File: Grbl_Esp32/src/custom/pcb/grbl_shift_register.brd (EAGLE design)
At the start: 69 parts

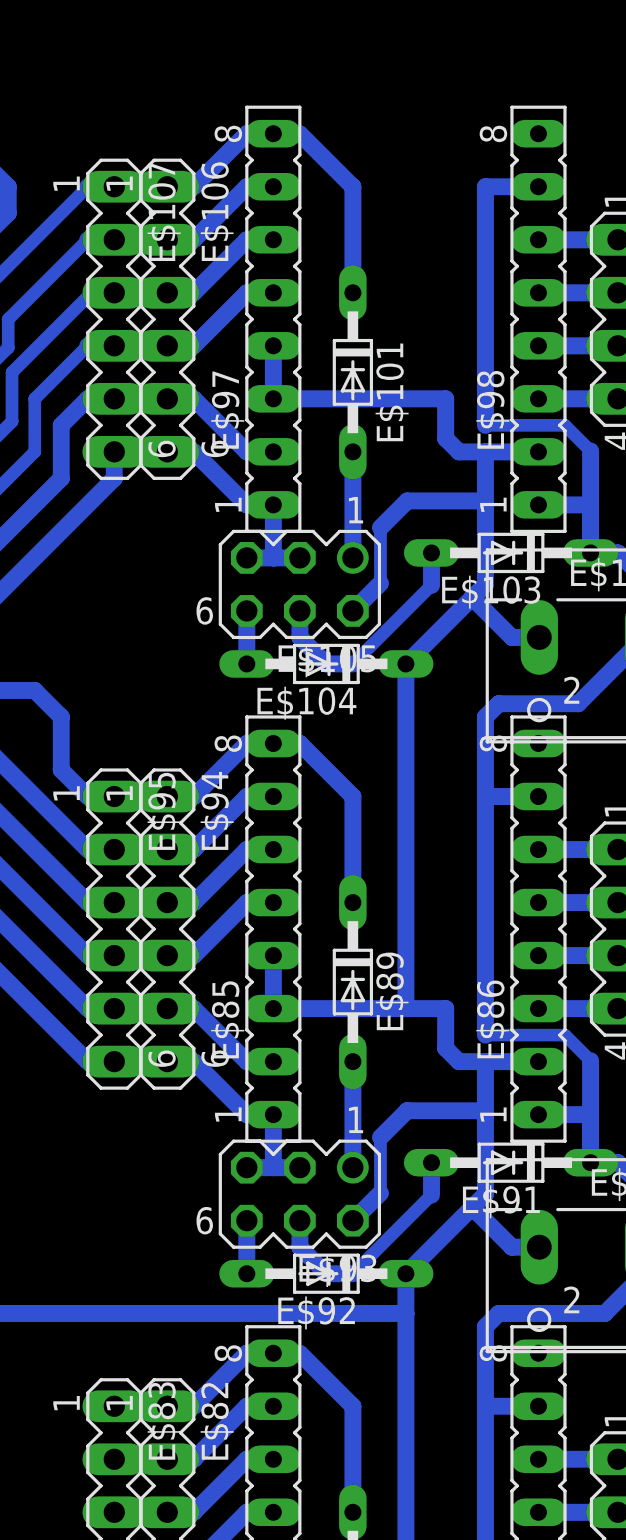
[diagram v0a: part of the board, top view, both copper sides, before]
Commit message: pcb
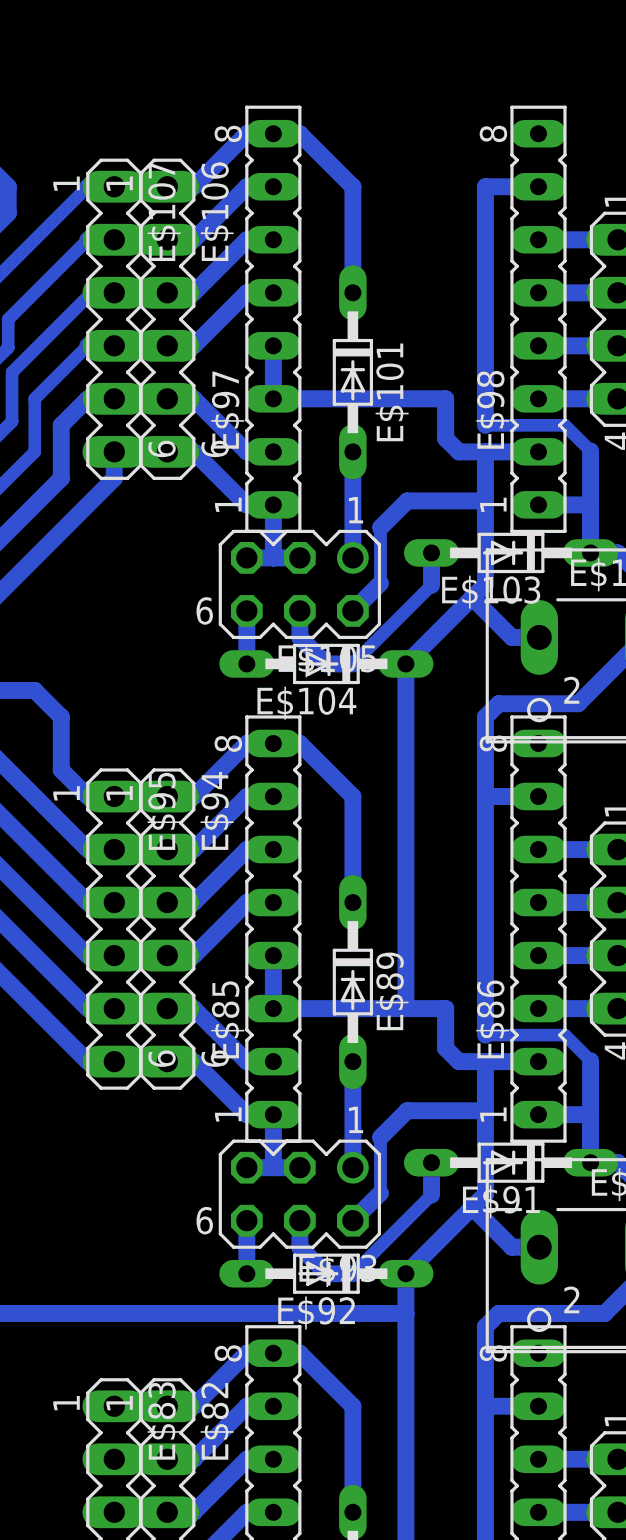
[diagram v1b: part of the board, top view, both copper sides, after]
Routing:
- net S$89: track 17.3 -> 18.6 mm
- net S$115: track 30.7 -> 32.0 mm
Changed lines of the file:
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@@
 <contactref element="E$77" pad="C"/>
 <contactref element="E$73" pad="8"/>
-<wire x1="83.82" y1="26.67" x2="81.28" y2="29.21" width="0.8128" layer="16"/>
+<wire x1="81.28" y1="29.21" x2="83.82" y2="26.67" width="0.8128" layer="16"/>
 <wire x1="83.82" y1="26.67" x2="83.82" y2="21.59" width="0.8128" layer="16"/>
 <contactref element="E$82" pad="1"/>
@@
 <wire x1="76.2" y1="26.67" x2="74.93" y2="26.67" width="0.8128" layer="16"/>
 <wire x1="74.93" y1="26.67" x2="72.39" y2="26.67" width="0.8128" layer="16"/>
+<wire x1="80.01" y1="29.21" x2="81.28" y2="29.21" width="0.8128" layer="16"/>
 </signal>
 <signal name="S$90">
@@
 <contactref element="E$101" pad="C"/>
 <contactref element="E$97" pad="8"/>
-<wire x1="83.82" y1="85.09" x2="81.28" y2="87.63" width="0.8128" layer="16"/>
+<wire x1="81.28" y1="87.63" x2="83.82" y2="85.09" width="0.8128" layer="16"/>
 <wire x1="83.82" y1="85.09" x2="83.82" y2="80.01" width="0.8128" layer="16"/>
 <contactref element="E$106" pad="1"/>
@@
 <wire x1="63.5" y1="76.2" x2="63.58989375" y2="76.2" width="0.8128" layer="16"/>
 <wire x1="66.04" y1="78.65010625" x2="66.04" y2="80.01" width="0.6096" layer="16"/>
-<wire x1="80.01" y1="87.63" x2="81.28" y2="87.63" width="0" layer="19" extent="16-16"/>
+<wire x1="80.01" y1="87.63" x2="81.28" y2="87.63" width="0.8128" layer="16"/>
 </signal>
 <signal name="S$116">
